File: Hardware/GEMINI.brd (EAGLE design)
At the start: 50.4 x 40.6 mm, 75 parts, among them IC2 LMV358IDGKR, J1 ZX62-B-5PA(33), T1 FDN340P, U1 ATMEGA32U4-XUMU

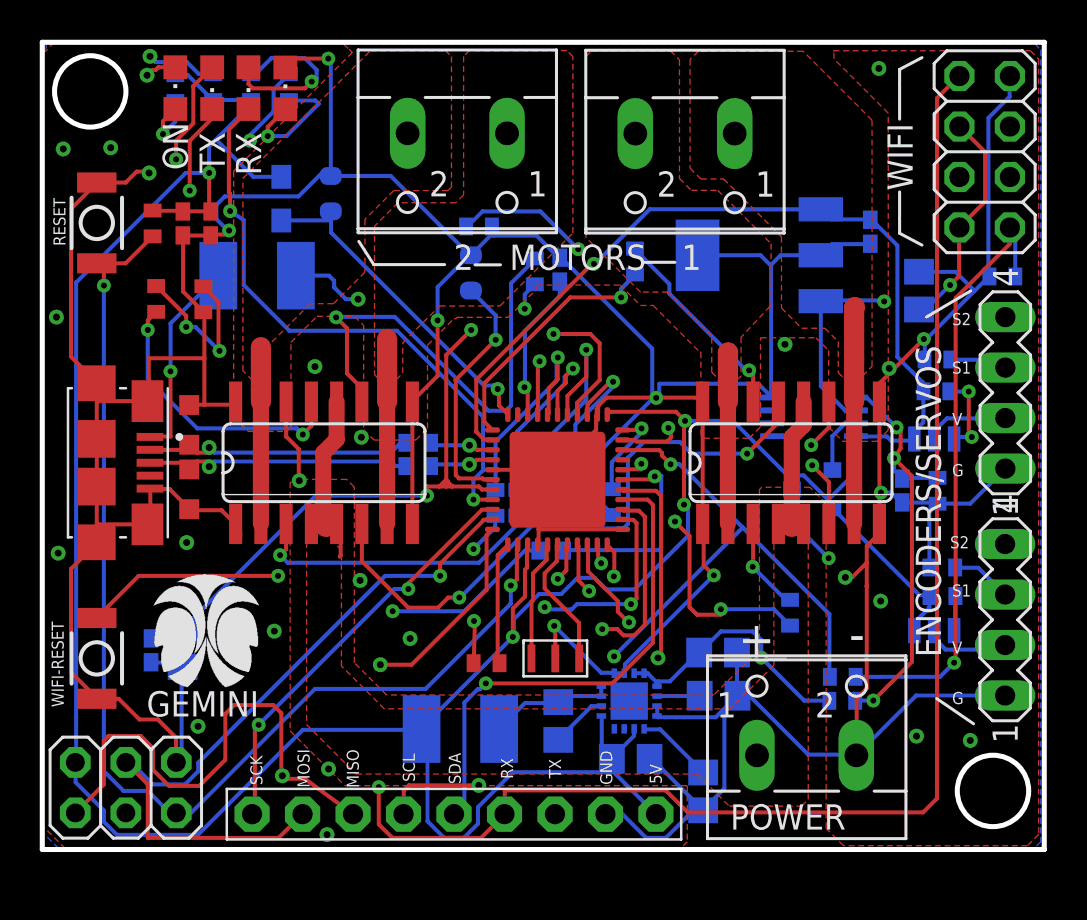
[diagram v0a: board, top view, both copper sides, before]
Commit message: gemini prod
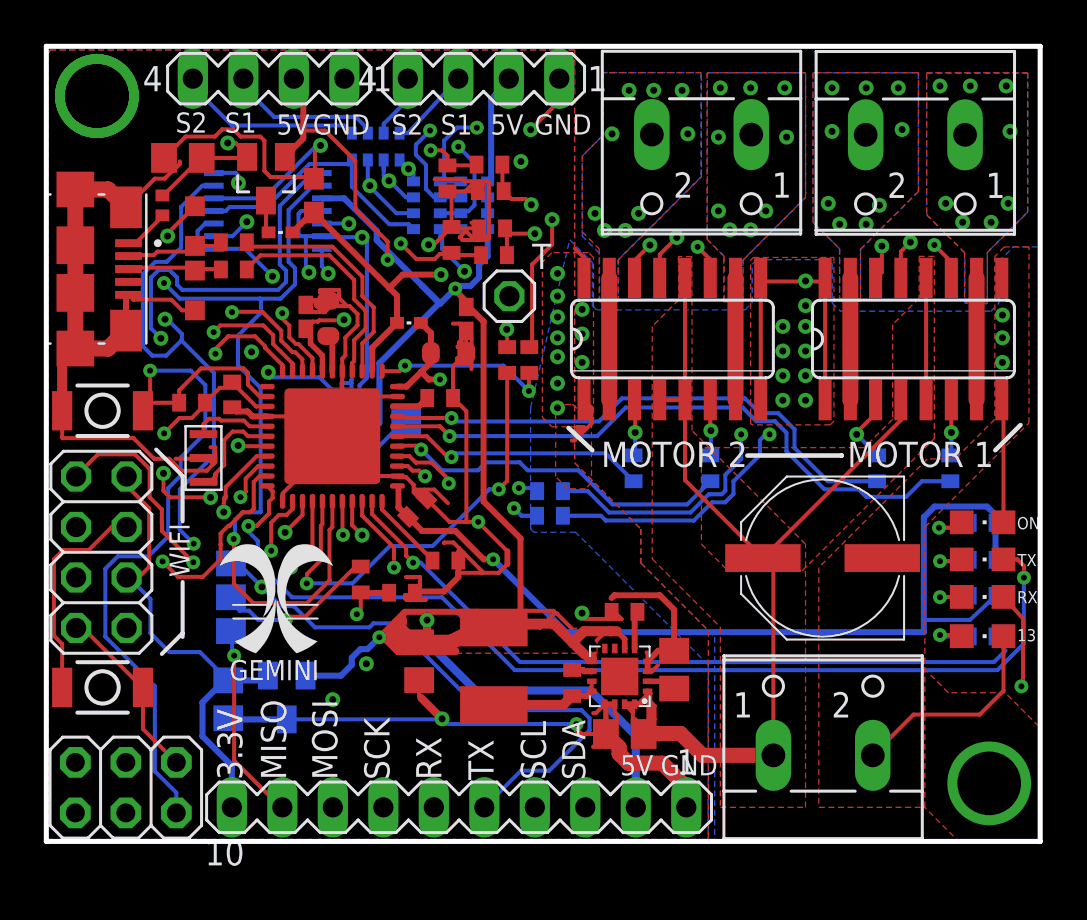
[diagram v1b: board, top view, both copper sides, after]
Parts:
- removed F1: MF-MSMF050-2 500mA, rcl:L1812
- removed IC1: (no value), linear-technology:SOT223
- removed IC2: LMV358IDGKR, linear:MSOP08
- removed JP1: (no value), adafruit:1X09-BIG
- removed R11, R13: 180, eagle-ltspice:R0402
- removed R12, R14: 10k, eagle-ltspice:R0402
- removed R15, R16: 2M, eagle-ltspice:R0402
- removed T1: FDN340P, zetex:SOT-23
- removed U$2, U$4: 2BRIDGE, 2BRIDGE:2BRIDGE
- added C12: (no value), rcl:PANASONIC_E
- added D3: SDM40E20LC-7, diode:SOT23
- added JMP1: 0R-JUMPB, jump-0r-smd:B0R-JMP
- added L2: MPZ1005A331ETD25, wuerth-elektronik:0402
- added LM2901AQT14-13: LM390, ds1803:TSSOP14
- added RN1: 10k, resistor-dil:CAT16
- added RN2: 3k, resistor-dil:CAT16
- added RN3: 10M, resistor-dil:CAT16
- added SV3: (no value), con-lstb:MA10-1
- added T: (no value), pinhead:1X01
- added U$5: MCP1812BT-3.3, ldo:SOT23
- added U$6: F0402E0R50FSTR, FUSE:R0402
- added VR1: 35WR10KLFTR, SamacSys_Parts:35WR100KLFTR
- C1: value 100n -> 2.2uF; device rcl:C0402K -> rcl:C0603
- C11, C6, C8: device rcl:C0402K -> rcl:C0402
- C37, C39: device rcl:C0805 -> rcl:C0402
- L1: value MH2029-300Y -> MPZ1005A331ETD25; device wuerth-elektronik:0805 -> wuerth-elektronik:0402
- LED: value Yellow -> BLUE
- moved JP5 48.8 mm to (2.77, 14.5), turned to 270 degrees
- moved R3 46.1 mm to (47.1, 16.0), turned to 0 degrees
- moved ON 46.1 mm to (47.1, 16.1), turned to 270 degrees
- moved TX 45.4 mm to (47.1, 14.2), turned to 270 degrees
- moved R7 45.4 mm to (47.1, 14.2), turned to 0 degrees
- moved RX 44.9 mm to (47.1, 12.3), turned to 270 degrees
- moved R6 44.8 mm to (47.1, 12.4), turned to 0 degrees
- moved LED 44.6 mm to (47.1, 10.3), turned to 270 degrees
- moved R1 44.5 mm to (47.1, 10.3), turned to 0 degrees
- moved C4 40.4 mm to (9.15, 7.15), turned to 270 degrees
- moved SV1 40.3 mm to (11.2, 38.4), turned to 180 degrees
- moved SV2 37.8 mm to (22.0, 38.4), turned to 180 degrees
- moved R8 34.1 mm to (17.9, 12.5), flipped to the top
- moved C1 33.1 mm to (13.5, 32.5), flipped to the top
- moved R2 24.7 mm to (15.8, 13.2), flipped to the top, turned to 270 degrees
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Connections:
- removed net +3.3V: C4.1, IC1.3, IC2.6, JP5.2, JP5.6
- removed net +5VF1: SV2.2, U$2.P$2
- removed net +5VF2: SV1.2, U$4.P$2
- removed net AGND: U1.43
- removed net CMP: C1.2, IC2.5, R12.1, R14.2
- removed net D0/RX: JP1.6, JP5.8, U1.25
- removed net D1/TX: JP1.7, R2.1, U1.31
- removed net F2_OUTA: SV2.4, U1.20
- removed net F2_OUTB: SV1.4, U1.21
- removed net F_OUTA: R15.1, SV2.3, U1.18
- removed net F_OUTB: R16.1, SV1.3, U1.19
- removed net GATE_CMD: IC2.7, T1.3
- new net +3V3: C4.1, JP5.2, JP5.6, SV3.10, U$5.1
- new net +5VP: C1.1, C11.1, C8.1, ICSP.2, L1.1, L2.2, R3.1, R4.2, R6.1, R7.1, U1.14, U1.2, U1.34
- new net E1I: RN1.8, SV2.3
- new net E1M: LM2901AQT14-13.1OUT, RN2.8, RN3.5, U1.20
- new net E2I: RN1.7, SV2.4
- new net E2M: LM2901AQT14-13.2OUT, RN2.7, RN3.6, U1.28
- new net E3I: RN1.6, SV1.3
- new net E3M: LM2901AQT14-13.3OUT, RN2.6, RN3.7, U1.21
- new net E4I: RN1.5, SV1.4
- new net E4M: LM2901AQT14-13.4OUT, RN2.5, RN3.8, U1.29
- new net N$22: LM2901AQT14-13.1IN-, LM2901AQT14-13.2IN-, LM2901AQT14-13.3IN-, LM2901AQT14-13.4IN-, T.1, VR1.2
- new net N$23: D3.3, L2.1
- new net N$25: JMP1.2, R2.1
- new net N$27: LM2901AQT14-13.2IN+, RN1.2, RN3.3
- new net N$28: LM2901AQT14-13.1IN+, RN1.1, RN3.4
- new net RX: SV3.6, U1.30
- new net TX: JMP1.3, SV3.5, U1.25
- new net WIFI-RX: JP5.8
- new net WIFI_RX: U1.12
- net +5V: now also D3.1, LM2901AQT14-13.VCC, RN2.1, RN2.2, RN2.3, RN2.4, SV1.2, SV2.2, SV3.2, U$5.2, VR1.1; no longer C11.1, C8.1, IC1.1, IC2.8, ICSP.2, JP1.9, L1.1, R11.1, R13.1, R3.1, R4.2, R6.1, R7.1, T1.2, U$2.P$3, U$4.P$3, U1.14, U1.2, U1.34
- net GND: now also C1.2, C12.-, LM2901AQT14-13.GND, SV3.1, U$5.3, U1.43, VR1.3; no longer C1.1, IC1.2, IC1.4, IC2.4, JP1.8, R14.1, R15.2, R16.2
- net M1_PWM: now also U1.26; no longer U1.12
- net M2_PWM: now also U1.31; no longer U1.29
- net M2_SEL: now also U1.27; no longer U1.28
- net MISO: now also JMP1.1, SV3.9; no longer JP1.3
- net MOSI: now also SV3.8; no longer JP1.2
- net N$2: now also LM2901AQT14-13.3IN+, RN1.3, RN3.2; no longer R11.2, U$2.P$1
- net N$3: now also LM2901AQT14-13.4IN+, RN1.4, RN3.1; no longer R13.2, U$4.P$1
- net SCK: now also SV3.7; no longer JP1.1
- net SCL: now also SV3.4, U1.18; no longer JP1.4, U1.27
- net SDA: now also SV3.3, U1.19; no longer JP1.5, U1.26
- net VIN: now also C12.+; no longer R12.2
- net VUSB: now also D3.2, U$6.2; no longer F1.1, T1.1
- net XUSB: now also U$6.1; no longer F1.2
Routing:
- net +5VP: track 0.00 -> 128.4 mm, vias 0 -> 3
- net D0/RX: track 94.1 -> 0.00 mm, vias 2 -> 0
- net E1M: track 0.00 -> 64.1 mm, vias 0 -> 4
- net +5V: track 196.5 -> 133.8 mm, vias 5 -> 4
- net E2M: track 0.00 -> 61.4 mm, vias 0 -> 3
- net E4M: track 0.00 -> 57.4 mm, vias 0 -> 4
- net N$22: track 0.00 -> 50.4 mm, vias 0 -> 4
- net E3M: track 0.00 -> 50.1 mm, vias 0 -> 3
- net RESET-WIFI: track 52.6 -> 11.0 mm, vias 1 -> 0
- net GND: track 307.5 -> 266.1 mm, vias 30 -> 35
- net D1/TX: track 35.4 -> 0.00 mm, vias 2 -> 0
- net TX: track 0.00 -> 34.7 mm, vias 0 -> 2
- net N$8: track 10.2 -> 42.5 mm, vias 1 -> 2
- net F_OUTB: track 31.1 -> 0.00 mm, vias 1 -> 0
- net F_OUTA: track 30.6 -> 0.00 mm, vias 1 -> 0
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- added copper zone on layer 1, net +5V
- added copper zone on layer 15, net GND
- added copper zone on layer 2, net GND
- added copper zone on layer 16, net MOT1_A
- added copper zone on layer 16, net MOT1_B
- added copper zone on layer 16, net MOT2_A
- added copper zone on layer 16, net MOT2_B
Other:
- board size 50.4 x 40.6 mm -> 50 x 40 mm
- board text added: "13"
- board text added: "3.3V"
- board text added: "C:/Users/franc/Desktop/palloncino.bmp"
- board text added: "MOTOR 1"
- board text added: "MOTOR 2"
- board text added: "ON"
- board text added: "OPEN-HARDWARE PLATFORM"
- board text added: "desigened by S.D/F.B/L.V"
- board text added: "designed by S.D/F.B/L.V"
- board text removed: "1"
- board text removed: "2"
- board text removed: "ENCODERS/SERVOS"
- board text removed: "G"
- board text removed: "MOTORS"
- board text removed: "RESET"
- board text removed: "SAMUELE "SAMIR" D'ANGELO FRANCESCO "C0BRA" BROCCA LUDOVICO "DEFALT" VIERO"
- board text removed: "V"
- board text removed: "WIFI-RESET"
